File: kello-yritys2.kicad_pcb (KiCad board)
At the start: 2 copper layers, 189.2 x 105.4 mm, 195 parts, among them J1 Conn_01x02_Male_To_Opto, J2 USB_B_Micro, J3 AVR-ISP-6, Q1 TEPT4400, Q10 BC850, Q11 BC850, Q12 BC850, Q13 BC850, Q14 BC850, Q15 BC850, Q16 BC850, Q17 BC850, Q18 BC850, Q19 BC850, Q2 IRLML6402, Q20 BC850, Q21 BC850, Q22 BC850, Q23 BC850, Q24 BC850, Q25 BC850, Q26 BC850, Q27 BC850, Q28 BC850, Q29 BC850, Q3 IRLML6402, Q30 BC850, Q31 BC850, Q32 BC850, Q33 BC850, Q4 IRLML6402, Q5 IRLML6402, Q6 BC850, Q7 BC850, Q8 BC850, Q9 BC850, SW1 SW_Push_Dual, SW2 SW_Push_Dual, U1 ATmega328PB-AU

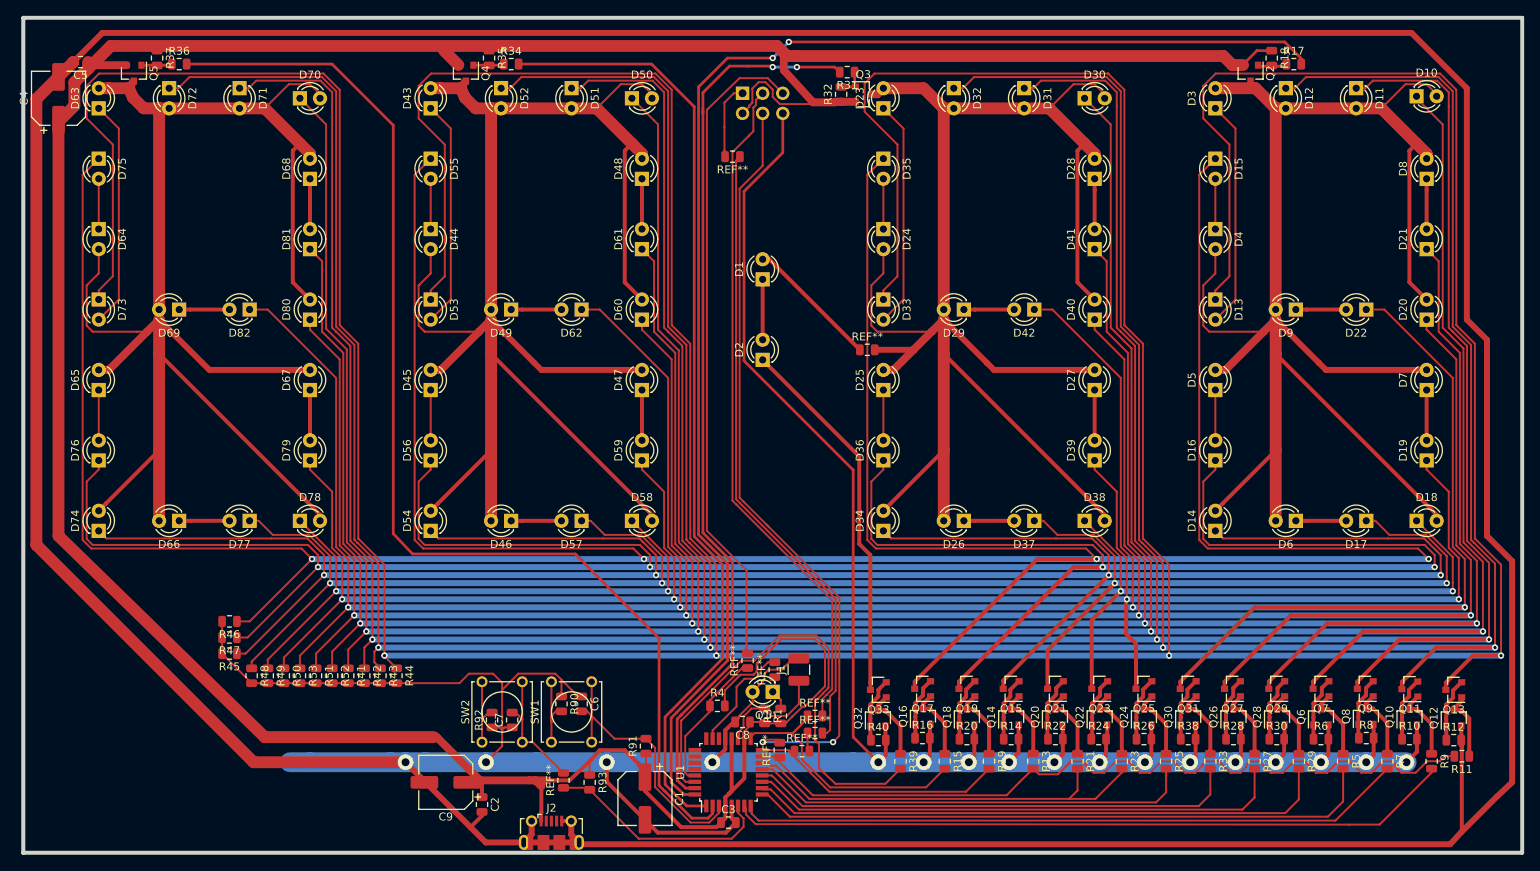
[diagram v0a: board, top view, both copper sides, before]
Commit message: joo
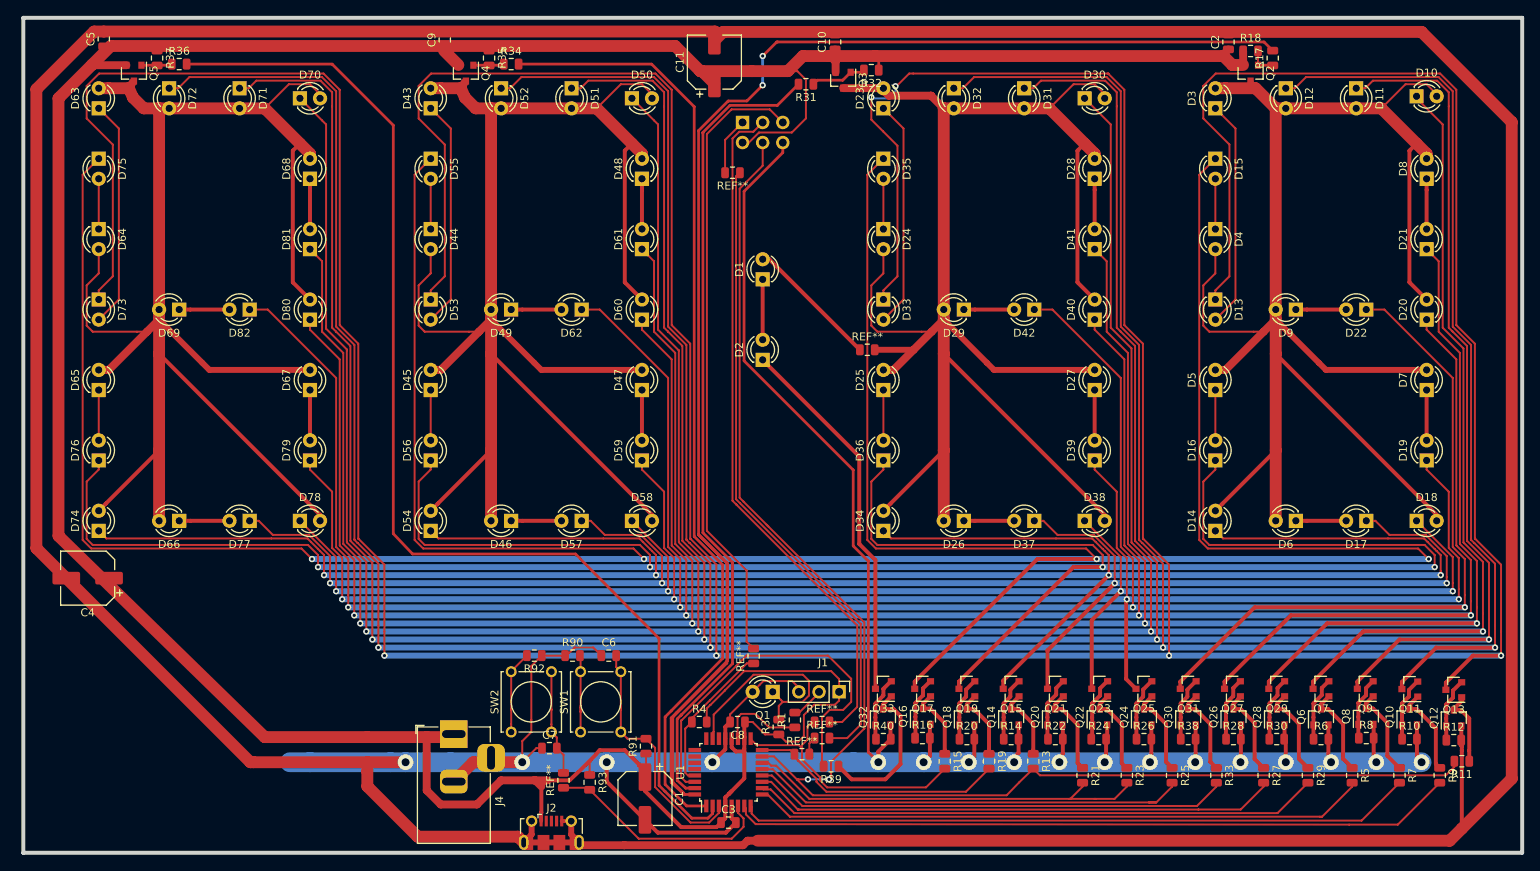
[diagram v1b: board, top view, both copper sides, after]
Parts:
- removed R41, R42, R43, R44, R45, R46, R47, R48, R49, R50, R51, R52, R53: 1M, Resistor_SMD:R_0805_2012Metric
- removed the REF** at (107.6, 93.7)
- removed the REF** at (108.2, 103.9)
- removed the REF** at (104.1, 92.6)
- removed the REF** at (111.0, 104.0)
- removed the REF** at (102.2, 29.0)
- removed the REF** at (112.6, 101.7)
- added C10: 100n, Capacitor_SMD:C_0805_2012Metric, F.Cu at (115.2, 14.5)
- added C11: 100u, Capacitor_SMD:CP_Elec_6.3x7.7, F.Cu at (99.9, 17.0)
- added J4: Barrel_Jack, Connector_BarrelJack:BarrelJack_Horizontal, F.Cu at (67.1, 101.9)
- added REF**: 0, Resistor_SMD:R_0805_2012Metric, F.Cu at (104.9, 92.0)
- added REF**: 0, Resistor_SMD:R_0805_2012Metric, F.Cu at (111.0, 104.4)
- added REF**: 0, Resistor_SMD:R_0805_2012Metric, F.Cu at (102.2, 31.0)
- added REF**: 0, Resistor_SMD:R_0805_2012Metric, F.Cu at (113.5, 102.4)
- C2: value 100nF -> 100n
- C9: value 100uF -> 100n; footprint Capacitor_SMD:CP_Elec_6.3x7.7 -> Capacitor_SMD:C_0805_2012Metric
- J1: footprint Resistor_SMD:R_1210_3225Metric -> Connector_PinHeader_2.54mm:PinHeader_1x03_P2.54mm_Vertical
- R1: value 47k -> 1k
- moved C2 134.7 mm to (164.8, 14.5), turned to 90 degrees
- moved C9 93.7 mm to (65.9, 14.2), turned to 90 degrees
- moved C4 60.7 mm to (20.8, 82.2), turned to 180 degrees
- moved R92 9.72 mm to (77.2, 91.9), turned to 180 degrees
- moved R39 8.79 mm to (114.7, 105.9), turned to 180 degrees
- moved C6 6.99 mm to (86.6, 91.9), turned to 0 degrees
- moved R90 6.25 mm to (82.0, 91.9), turned to 0 degrees
- moved C7 5.89 mm to (79.1, 103.6), turned to 0 degrees
- moved J1 5.80 mm to (115.7, 96.5), turned to 270 degrees
- moved R31 5.43 mm to (111.5, 19.8)
- moved R32 4.88 mm to (119.8, 18.0), turned to 180 degrees
- moved C5 4.13 mm to (22.9, 14.1), turned to 90 degrees
- moved SW1 3.90 mm to (83.1, 101.6)
- moved SW2 3.90 mm to (74.3, 101.6)
- moved R1 3.84 mm to (110.1, 100.1), turned to 90 degrees
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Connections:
- J1 pad 1: Net-(J1-Pad1) -> +5V
- J1 pad 2: Earth -> Net-(J1-Pad2)
- R1 pad 1: Net-(J1-Pad1) -> Net-(R1-Pad1)
- R1 pad 2: +5V -> Net-(J1-Pad2)
- U1 pad 19: Net-(J1-Pad1) -> Net-(R1-Pad1)
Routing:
- net Earth: track 976.3 -> 942.3 mm
- net /Naytto/Ghi0: track 175.7 -> 207.6 mm
- net /Naytto/Numero/Cat3b: track 306.4 -> 291.3 mm
- net /Naytto/Numero/Cat6a: track 234.4 -> 219.5 mm
- net Net-(J1-Pad1): track 14.5 -> 0.00 mm
- net /Naytto/Numero/Cat5: track 347.4 -> 333.4 mm
- net /Naytto/Glo3: track 200.4 -> 186.8 mm
- net /Naytto/Numero/Cat6b: track 211.3 -> 197.9 mm
- net /Naytto/Numero/Cat4: track 499.7 -> 487.0 mm
- net /Naytto/GloB: track 60.8 -> 48.8 mm
- net /Naytto/Numero/Cat7: track 241.4 -> 229.7 mm
- net Net-(R1-Pad1): track 0.00 -> 10.8 mm
- net Net-(Q32-Pad3): track 9.27 -> 20.0 mm
- net /Naytto/Numero/CatA: track 368.3 -> 358.0 mm
- net /Naytto/Ghi1: track 113.1 -> 103.5 mm, vias 2 -> 0
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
